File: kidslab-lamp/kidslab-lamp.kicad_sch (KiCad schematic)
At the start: 38 parts, among them U1 Pico

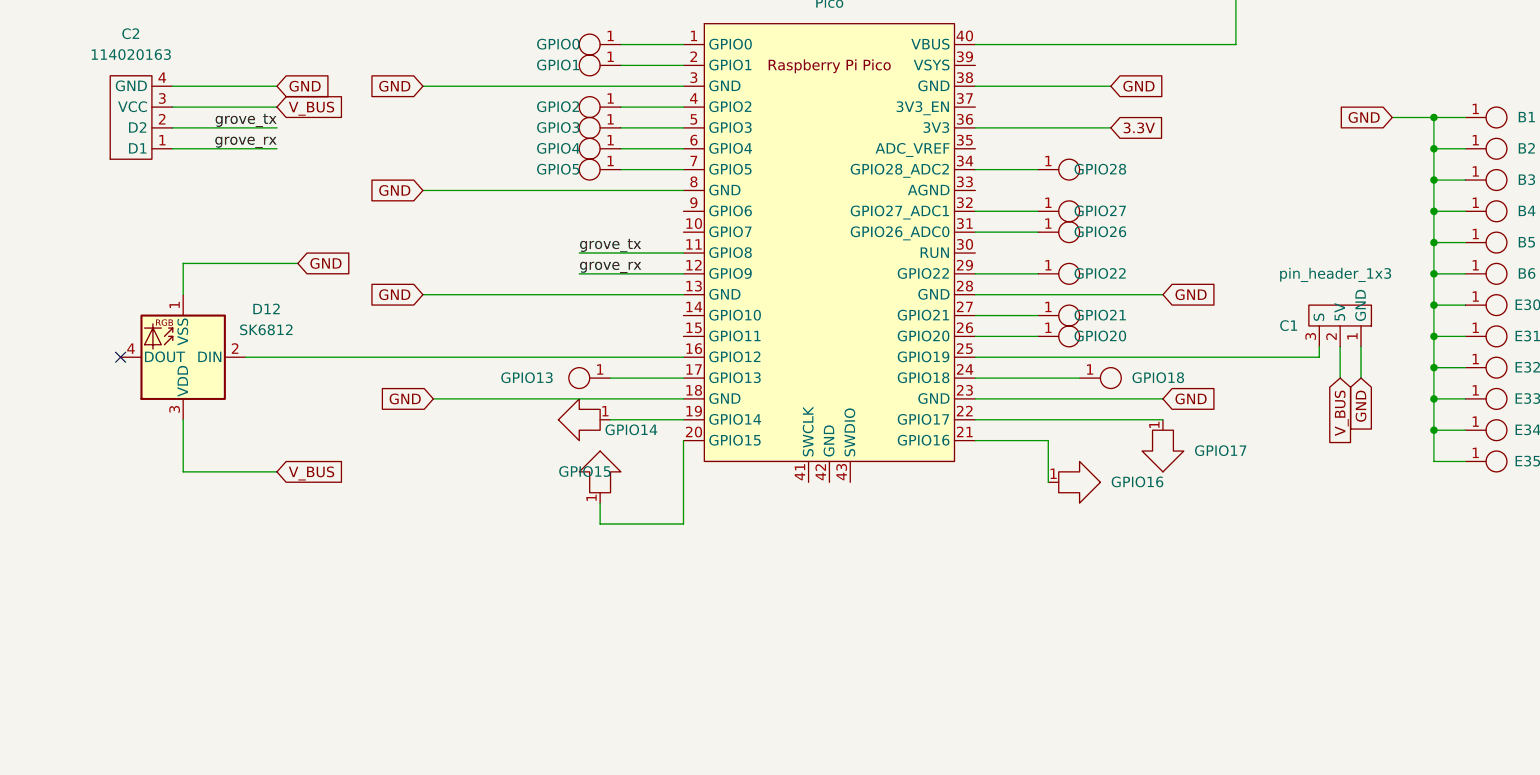
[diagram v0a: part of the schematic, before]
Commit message: updated PCB with requested changes
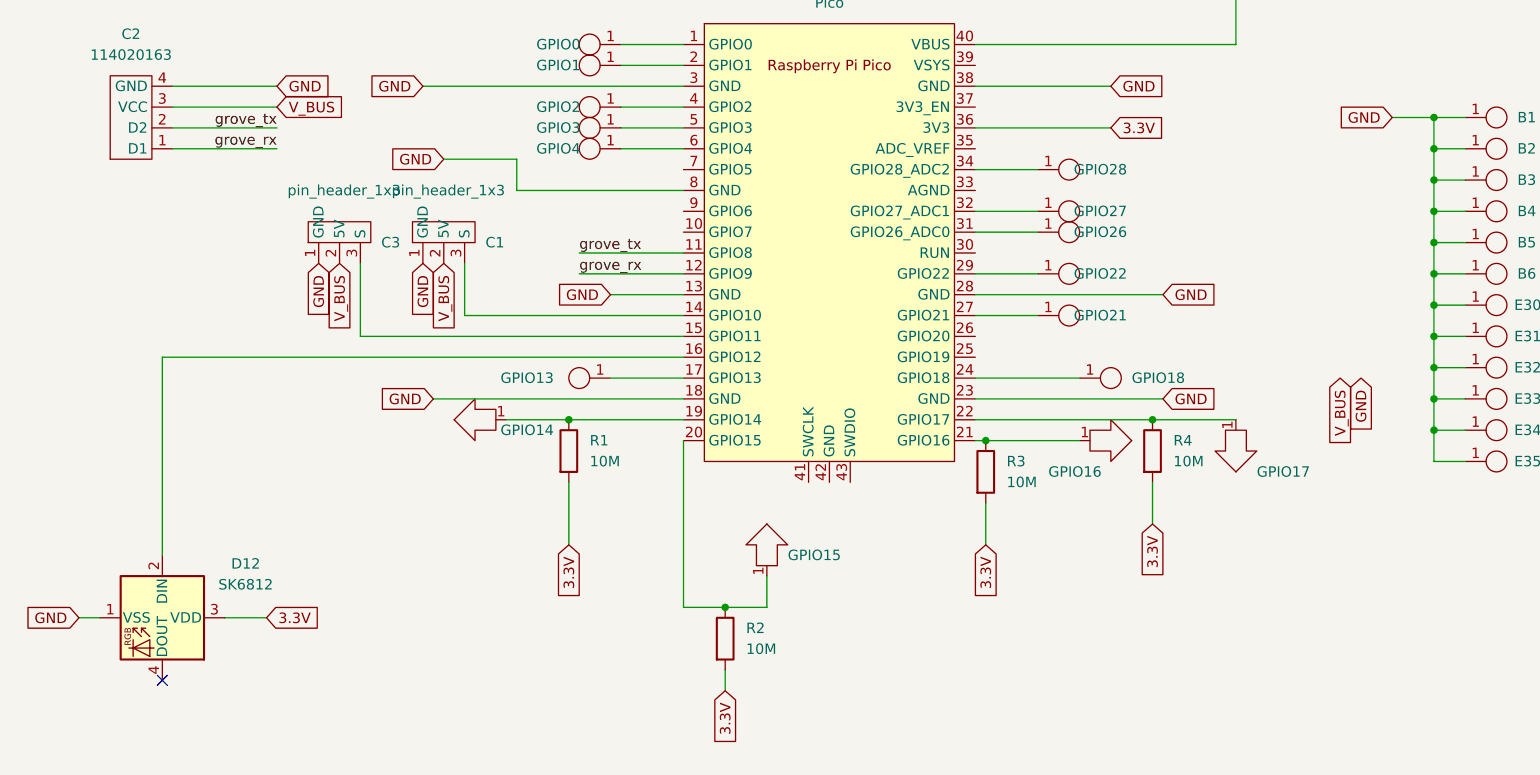
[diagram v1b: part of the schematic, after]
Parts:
- removed GPIO20, GPIO5: kroko_edge, kidslab:Edgeconnector, symbol kidslab:kroko_edge
- added C3: pin_header_1x3, Connector_PinHeader_2.54mm:PinHeader_1x03_P2.54mm_Vertical, symbol kidslab:pin_header_1x3
- added R1, R2, R3, R4: 10M, Resistor_THT:R_Axial_DIN0204_L3.6mm_D1.6mm_P5.08mm_Horizontal, symbol Device:R
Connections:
- net 3.3V: now also D12.3 (VDD), R1.2, R2.2, R3.2, R4.2
- net GND: now also C3.1 (GND)
- net V_BUS: now also C3.2 (5V); no longer D12.3 (VDD)
- net at U1.14 (GPIO10): now also C1.3 (S)
- net at U1.15 (GPIO11): now also C3.3 (S)
- net at GPIO14.1, U1.19 (GPIO14): now also R1.1
- net at GPIO15.1, U1.20 (GPIO15): now also R2.1
- net at GPIO16.1, U1.21 (GPIO16): now also R3.1
- net at GPIO17.1, U1.22 (GPIO17): now also R4.1
- net at U1.25 (GPIO19): no longer C1.3 (S)
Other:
- moved on the sheet: C1, D12, GPIO14, GPIO15, GPIO16, GPIO17

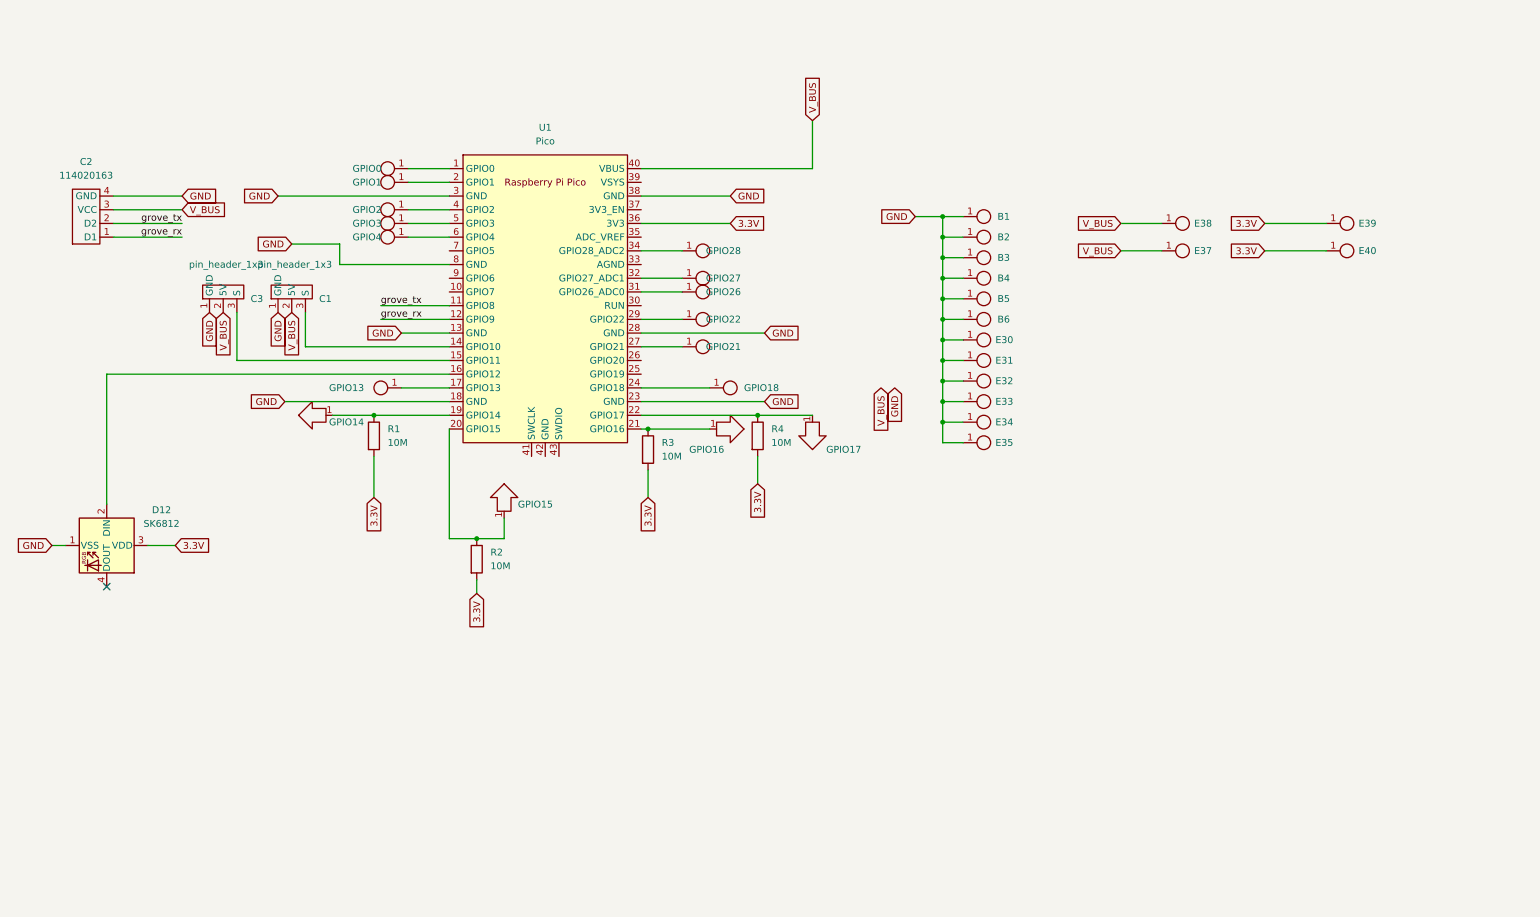
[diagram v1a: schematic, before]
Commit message: cleared schematics and exported pdf, fixed some routing issues, generated gerber files
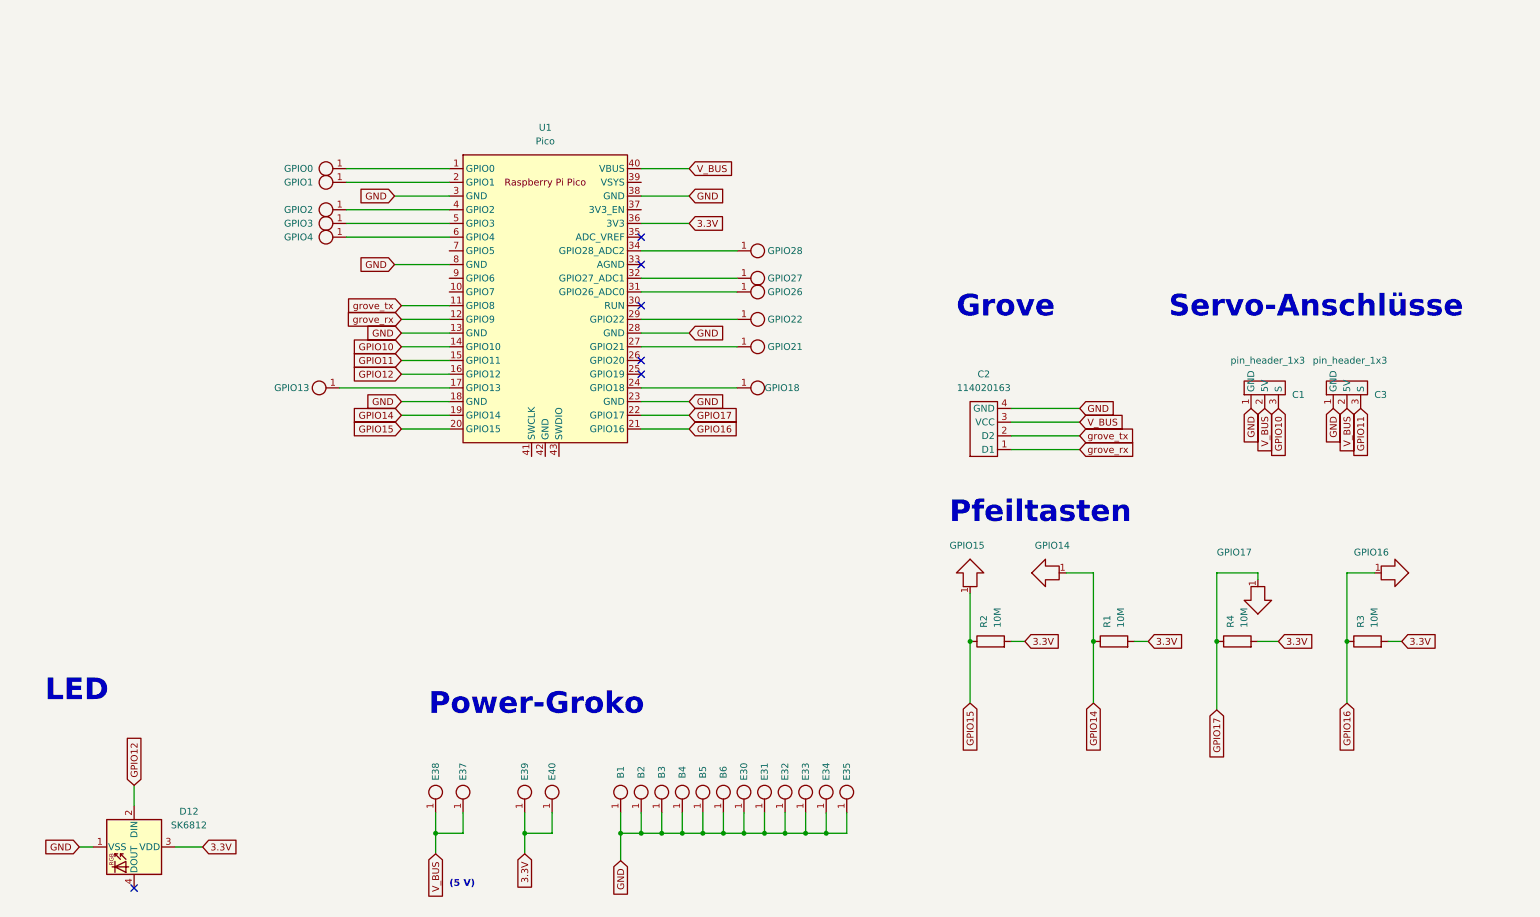
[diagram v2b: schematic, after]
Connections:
- net GPIO11: now reaches C3.3 (S), U1.15 (GPIO11)
- net GPIO16: now reaches GPIO16.1, R3.1, U1.21 (GPIO16)
- net GPIO10: now reaches C1.3 (S), U1.14 (GPIO10)
- net GPIO12: now reaches D12.2 (DIN), U1.16 (GPIO12)
- net GPIO14: now reaches GPIO14.1, R1.1, U1.19 (GPIO14)
- net GPIO15: now reaches GPIO15.1, R2.1, U1.20 (GPIO15)
- net GPIO17: now reaches GPIO17.1, R4.1, U1.22 (GPIO17)
- no-connect marks 1 -> 6
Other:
- note added: "(5 V)"
- note added: "Grove"
- note added: "LED"
- note added: "Pfeiltasten"
- note added: "Power-Groko"
- note added: "Servo-Anschlüsse"
- moved on the sheet: B1, B2, B3, B4, B5, B6, C1, C2, C3, D12, E30, E31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

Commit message: adding components to schematic
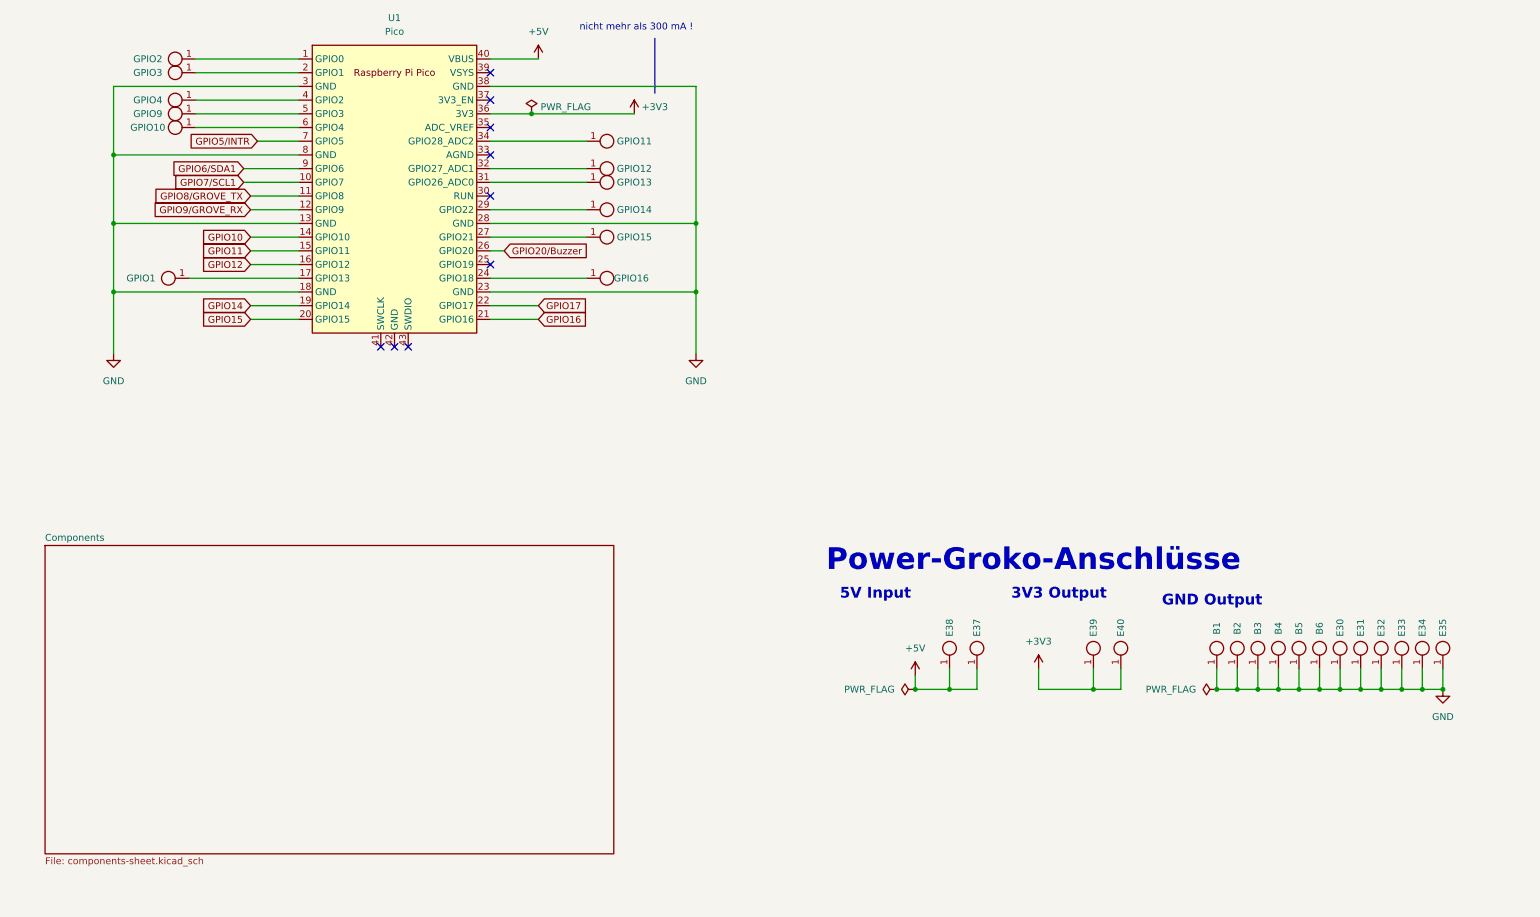
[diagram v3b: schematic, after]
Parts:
- removed C1, C3: pin_header_1x3, Connector_PinHeader_2.54mm:PinHeader_1x03_P2.54mm_Vertical, symbol kidslab:pin_header_1x3
- removed C2: 114020163, kidslab:114020163, symbol kidslab:114020163
- removed D12: SK6812, LED_SMD:LED_SK6812_PLCC4_5.0x5.0mm_P3.2mm, symbol LED:SK6812
- removed GPIO0, GPIO1, GPIO21, GPIO22, GPIO26, GPIO27, GPIO28: kroko_edge, kidslab:Edgeconnector, symbol kidslab:kroko_edge
- removed GPIO13, GPIO18: kroko_board, kidslab:KrokoConnector, symbol kidslab:kroko_board
- removed GPIO14, GPIO15, GPIO16, GPIO17: arrow, kidslab:Kroko_Arrow, symbol kidslab:arrow
- removed R1, R2, R3, R4: 10M, Resistor_THT:R_Axial_DIN0204_L3.6mm_D1.6mm_P5.08mm_Horizontal, symbol Device:R
- added GPIO1, GPIO16: kroko_board, kidslab:KrokoConnector, symbol kidslab:kroko_board
- added GPIO10, GPIO11, GPIO12, GPIO13, GPIO14, GPIO15, GPIO9: kroko_edge, kidslab:Edgeconnector, symbol kidslab:kroko_edge
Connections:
- net at U1.24 (GPIO18): now also GPIO16.1
- net at U1.29 (GPIO22): now also GPIO14.1
- net at U1.1 (GPIO0): now also GPIO2.1
- net GPIO7/SCL1: now reaches U1.10 (GPIO7)
- net at U1.17 (GPIO13): now also GPIO1.1
- net at U1.2 (GPIO1): now also GPIO3.1
- net GPIO20/Buzzer: now reaches U1.26 (GPIO20)
- net at U1.27 (GPIO21): now also GPIO15.1
- net at U1.31 (GPIO26_ADC0): now also GPIO13.1
- net at U1.32 (GPIO27_ADC1): now also GPIO12.1
- net at U1.34 (GPIO28_ADC2): now also GPIO11.1
- net at U1.4 (GPIO2): now also GPIO4.1; no longer GPIO2.1
- net at U1.5 (GPIO3): now also GPIO9.1; no longer GPIO3.1
- net at U1.6 (GPIO4): now also GPIO10.1; no longer GPIO4.1
- net GPIO5/INTR: now reaches U1.7 (GPIO5)
- net GPIO6/SDA1: now reaches U1.9 (GPIO6)
- net 3.3V renamed +3V3
- net V_BUS renamed +5V
- net grove_rx renamed GPIO9/GROVE_RX
- net grove_tx renamed GPIO8/GROVE_TX
- no-connect marks 6 -> 9
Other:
- added sheet Components (components-sheet.kicad_sch)
- note added: "3V3 Output"
- note added: "5V Input"
- note added: "GND Output"
- note added: "Power-Groko-Anschlüsse"
- note added: "nicht mehr als 300 mA !"
- note removed: "(5 V)"
- note removed: "Grove"
- note removed: "LED"
- note removed: "Pfeiltasten"
- note removed: "Power-Groko"
- note removed: "Servo-Anschlüsse"
- moved on the sheet: B1, B2, B3, B4, B5, B6, E30, E31, E32, E33, E34, E35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
